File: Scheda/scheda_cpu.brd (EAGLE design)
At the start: 90 x 70 mm, 47 parts, among them IC2 LM380, IC3 AMS1117-3.3V, T1 BC-817, T2 MCU80N03A, T3 MCU80N03A, T4 MCU80N03A, T5 MCU80N03A

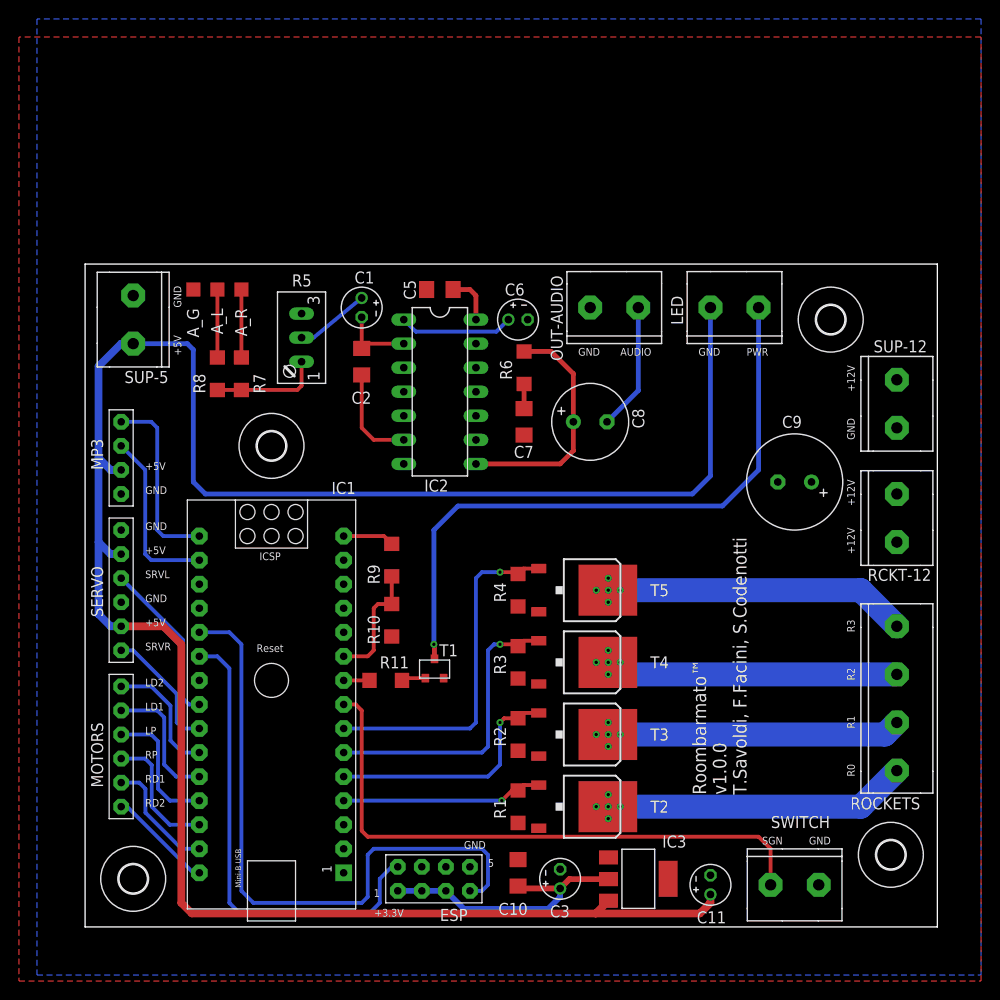
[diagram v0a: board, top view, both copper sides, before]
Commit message: completato PCB
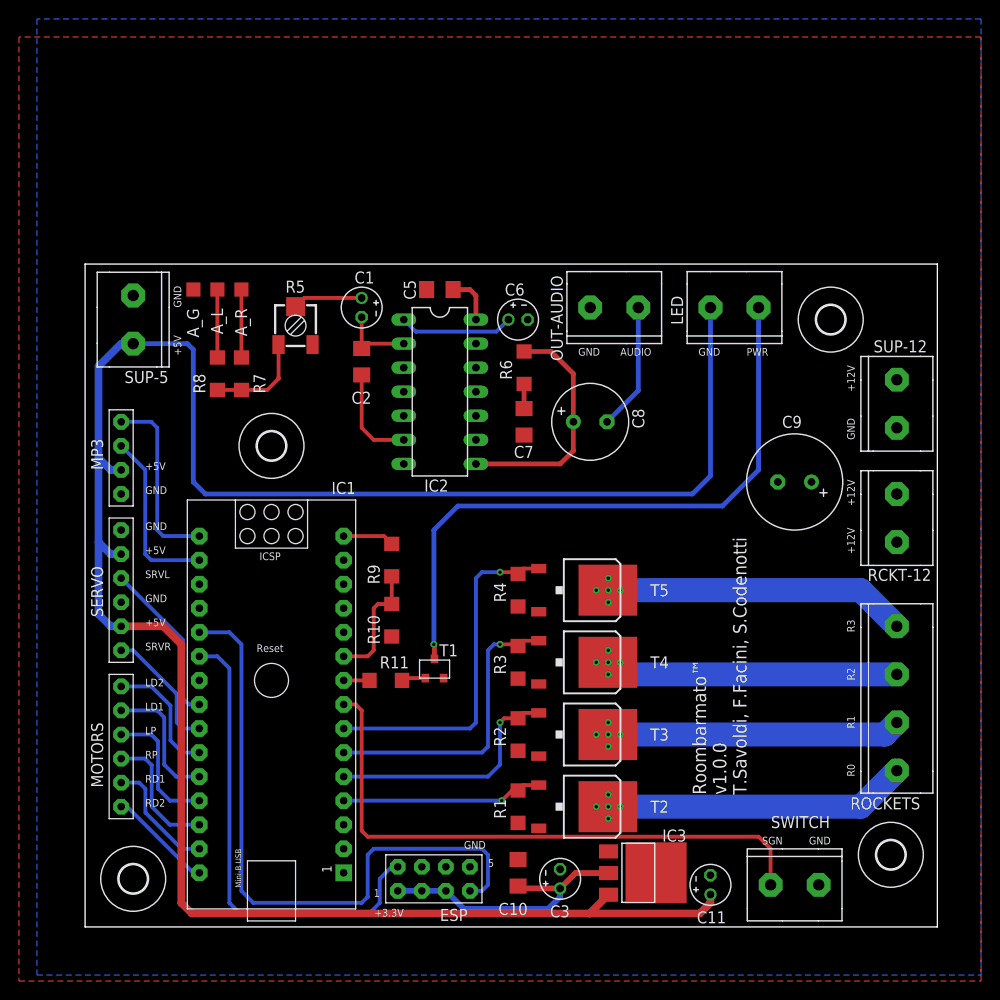
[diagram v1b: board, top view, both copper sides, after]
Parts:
- R5: value 100k -> 50k; device pot:S64W -> rcl:RTRIM3314J
- moved R5 1.42 mm to (22.2, 63.5), turned to 0 degrees
- moved IC3 0.63 mm to (58.4, 5.71)
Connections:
- net GND: now also R5.1; no longer R5.E
- net IN_AUDIO: now also R5.3; no longer R5.A
- net N$5: now also R5.2; no longer R5.S
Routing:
- net IN_AUDIO: track 11.6 -> 10.6 mm
- net +5V: track 227.9 -> 228.8 mm
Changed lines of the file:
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@@
 <grid distance="25" unitdist="mil" unit="mil" style="lines" multiple="1" display="yes" altdistance="5" altunitdist="mil" altunit="mil"/>
 <layers>
-<layer number="1" name="Top" color="4" fill="1" visible="no" active="yes"/>
-<layer number="16" name="Bottom" color="1" fill="1" visible="no" active="yes"/>
+<layer number="1" name="Top" color="4" fill="1" visible="yes" active="yes"/>
+<layer number="16" name="Bottom" color="1" fill="1" visible="yes" active="yes"/>
 <layer number="17" name="Pads" color="2" fill="1" visible="yes" active="yes"/>
 <layer number="18" name="Vias" color="2" fill="1" visible="yes" active="yes"/>
@@
 <layer number="25" name="tNames" color="7" fill="1" visible="yes" active="yes"/>
 <layer number="26" name="bNames" color="7" fill="1" visible="yes" active="yes"/>
-<layer number="27" name="tValues" color="7" fill="1" visible="yes" active="yes"/>
-<layer number="28" name="bValues" color="7" fill="1" visible="yes" active="yes"/>
-<layer number="29" name="tStop" color="7" fill="3" visible="yes" active="yes"/>
-<layer number="30" name="bStop" color="7" fill="6" visible="yes" active="yes"/>
+<layer number="27" name="tValues" color="7" fill="1" visible="no" active="yes"/>
+<layer number="28" name="bValues" color="7" fill="1" visible="no" active="yes"/>
+<layer number="29" name="tStop" color="7" fill="3" visible="no" active="yes"/>
+<layer number="30" name="bStop" color="7" fill="6" visible="no" active="yes"/>
 <layer number="31" name="tCream" color="7" fill="4" visible="no" active="yes"/>
 <layer number="32" name="bCream" color="7" fill="5" visible="no" active="yes"/>
@@
 <layer number="42" name="bRestrict" color="1" fill="10" visible="yes" active="yes"/>
 <layer number="43" name="vRestrict" color="2" fill="10" visible="no" active="yes"/>
-<layer number="44" name="Drills" color="7" fill="1" visible="yes" active="yes"/>
+<layer number="44" name="Drills" color="7" fill="1" visible="no" active="yes"/>
 <layer number="45" name="Holes" color="7" fill="1" visible="no" active="yes"/>
 <layer number="46" name="Milling" color="3" fill="1" visible="no" active="yes"/>
@@
 <text x="40.005" y="8.255" size="0.8128" layer="25">GND</text>
 <text x="81.28" y="31.115" size="0.8128" layer="25" rot="R90">R3</text>
-<polygon width="0.1524" layer="17">
-<vertex x="57.785" y="7.62"/>
-<vertex x="57.785" y="2.54"/>
-<vertex x="63.5" y="2.54"/>
-<vertex x="63.5" y="7.62"/>
-</polygon>
 <text x="52.07" y="60.325" size="0.8128" layer="25">GND</text>
 <text x="64.77" y="60.325" size="0.8128" layer="25">GND</text>
@@
 <attribute name="NAME" x="35.814" y="45.974" size="1.27" layer="25" ratio="10"/>
 </element>
-<element name="R5" library="pot" library_urn="urn:adsk.eagle:library:331" package="S64W" package3d_urn="urn:adsk.eagle:package:22708/1" value="100k" x="21.59" y="62.23" smashed="yes" rot="R270">
-<attribute name="NAME" x="21.844" y="67.6402" size="1.27" layer="25" ratio="10"/>
-<attribute name="POPULARITY" value="4" x="21.59" y="62.23" size="1.778" layer="27" rot="R270" display="off"/>
+<element name="R5" library="rcl" library_urn="urn:adsk.eagle:library:334" package="RTRIM3314J" package3d_urn="urn:adsk.eagle:package:26019/1" value="50k" x="22.225" y="63.5" smashed="yes">
+<attribute name="NAME" x="23.241" y="68.2498" size="1.27" layer="25" ratio="10" rot="R180"/>
+<attribute name="POPULARITY" value="0" x="22.225" y="63.5" size="1.778" layer="27" display="off"/>
+<attribute name="SPICEMODEL" value="X" x="22.225" y="63.5" size="1.778" layer="27" display="off"/>
+<attribute name="SPICEPREFIXL" value="POT" x="22.225" y="63.5" size="1.778" layer="27" display="off"/>
 </element>
 <element name="C1" library="ITIS" package="E2-4" value="10uF" x="29.21" y="65.405" smashed="yes" rot="R270">
@@
 </element>
 <element name="H4" library="ITIS" package="3,0" value="MOUNT-HOLE3.0" x="85.09" y="7.62" smashed="yes"/>
-<element name="IC3" library="roombarmato_eagle_lib" package="SOT223" package3d_urn="urn:adsk.eagle:package:4940/1" value="AMS1117-3.3V" x="58.42" y="5.08" smashed="yes" rot="R270">
-<attribute name="MF" value="" x="58.42" y="5.08" size="1.778" layer="27" rot="R270" display="off"/>
-<attribute name="MPN" value="REG1117" x="58.42" y="5.08" size="1.778" layer="27" rot="R270" display="off"/>
-<attribute name="NAME" x="63.5" y="9.652" size="1.27" layer="25" ratio="10" rot="R180"/>
-<attribute name="OC_FARNELL" value="1097566" x="58.42" y="5.08" size="1.778" layer="27" rot="R270" display="off"/>
-<attribute name="OC_NEWARK" value="14P6981" x="58.42" y="5.08" size="1.778" layer="27" rot="R270" display="off"/>
-<attribute name="POPULARITY" value="49" x="58.42" y="5.08" size="1.778" layer="27" rot="R270" display="off"/>
+<element name="IC3" library="roombarmato_eagle_lib" package="SOT223" package3d_urn="urn:adsk.eagle:package:4940/1" value="AMS1117-3.3V" x="58.42" y="5.715" smashed="yes" rot="R270">
+<attribute name="MF" value="" x="58.42" y="5.715" size="1.778" layer="27" rot="R270" display="off"/>
+<attribute name="MPN" value="REG1117" x="58.42" y="5.715" size="1.778" layer="27" rot="R270" display="off"/>
+<attribute name="NAME" x="63.5" y="10.287" size="1.27" layer="25" ratio="10" rot="R180"/>
+<attribute name="OC_FARNELL" value="1097566" x="58.42" y="5.715" size="1.778" layer="27" rot="R270" display="off"/>
+<attribute name="OC_NEWARK" value="14P6981" x="58.42" y="5.715" size="1.778" layer="27" rot="R270" display="off"/>
+<attribute name="POPULARITY" value="49" x="58.42" y="5.715" size="1.778" layer="27" rot="R270" display="off"/>
 </element>
 <element name="C10" library="ITIS" package="C1206" value="100nF" x="45.72" y="5.715" smashed="yes" rot="R90">
@@
 <contactref element="R1" pad="P$1"/>
 <contactref element="IC2" pad="5"/>
-<contactref element="R5" pad="E"/>
+<contactref element="R5" pad="1"/>
 <contactref element="C6" pad="-"/>
 <contactref element="C5" pad="2"/>
@@
 <wire x1="10.16" y1="2.54" x2="11.2776" y2="1.4224" width="0.8128" layer="1"/>
 <contactref element="IC3" pad="3"/>
-<wire x1="55.2704" y1="2.7686" x2="53.9242" y2="1.4224" width="0.8128" layer="1"/>
-<wire x1="11.2776" y1="1.4224" x2="53.9242" y2="1.4224" width="0.8128" layer="1"/>
-<wire x1="53.9242" y1="1.4224" x2="64.9224" y2="1.4224" width="0.8128" layer="1"/>
+<wire x1="55.2704" y1="3.4036" x2="53.2892" y2="1.4224" width="0.8128" layer="1"/>
+<wire x1="11.2776" y1="1.4224" x2="53.2892" y2="1.4224" width="0.8128" layer="1"/>
+<wire x1="53.2892" y1="1.4224" x2="64.9224" y2="1.4224" width="0.8128" layer="1"/>
 <contactref element="C11" pad="+"/>
 <wire x1="64.9224" y1="1.4224" x2="66.04" y2="2.54" width="0.8128" layer="1"/>
@@
 <contactref element="IC3" pad="2"/>
 <wire x1="40.005" y1="1.905" x2="48.895" y2="1.905" width="0.6096" layer="16"/>
-<wire x1="51.1556" y1="5.0546" x2="55.2704" y2="5.0546" width="0.6096" layer="1"/>
+<wire x1="51.7906" y1="5.6896" x2="55.2704" y2="5.6896" width="0.6096" layer="1"/>
 <contactref element="C10" pad="1"/>
 <contactref element="C3" pad="+"/>
-<wire x1="50.165" y1="4.064" x2="51.1556" y2="5.0546" width="0.6096" layer="1"/>
+<wire x1="50.165" y1="4.064" x2="51.7906" y2="5.6896" width="0.6096" layer="1"/>
 <wire x1="48.895" y1="1.905" x2="50.165" y2="3.175" width="0.6096" layer="16"/>
 <wire x1="50.165" y1="3.175" x2="50.165" y2="4.064" width="0.6096" layer="16"/>
@@
 </signal>
 <signal name="IN_AUDIO">
-<contactref element="R5" pad="A"/>
+<contactref element="R5" pad="3"/>
 <contactref element="R7" pad="P$2"/>
 <contactref element="R8" pad="P$2"/>
-<wire x1="22.86" y1="57.15" x2="22.4155" y2="56.7055" width="0.4064" layer="1"/>
-<wire x1="22.86" y1="57.15" x2="22.86" y2="59.69" width="0.4064" layer="1"/>
-<wire x1="22.4155" y1="56.7055" x2="16.51" y2="56.7055" width="0.4064" layer="1"/>
+<wire x1="20.45055625" y1="57.91555625" x2="19.2405" y2="56.7055" width="0.4064" layer="1"/>
+<wire x1="20.45055625" y1="57.91555625" x2="20.425" y2="57.9612125" width="0.4064" layer="1"/>
+<wire x1="20.425" y1="57.9612125" x2="20.425" y2="61.5" width="0.4064" layer="1"/>
+<wire x1="19.2405" y1="56.7055" x2="16.51" y2="56.7055" width="0.4064" layer="1"/>
 <wire x1="16.51" y1="56.7055" x2="13.97" y2="56.7055" width="0.4064" layer="1"/>
 </signal>
 <signal name="N$5">
-<contactref element="R5" pad="S"/>
+<contactref element="R5" pad="2"/>
 <contactref element="C1" pad="+"/>
-<wire x1="29.21" y1="66.421" x2="24.13" y2="62.23" width="0.4064" layer="16"/>
-<wire x1="22.86" y1="62.23" x2="24.13" y2="62.23" width="0.4064" layer="16"/>
+<wire x1="22.225" y1="65.5" x2="23.146" y2="66.421" width="0.4064" layer="1"/>
+<wire x1="23.146" y1="66.421" x2="29.21" y2="66.421" width="0.4064" layer="1"/>
 </signal>
 <signal name="N$6">
@@
 </signals>
 <mfgpreviewcolors>
-<mfgpreviewcolor name="soldermaskcolor" color="0xC8008000"/>
+<mfgpreviewcolor name="soldermaskcolor" color="0xC8FF00FF"/>
 <mfgpreviewcolor name="silkscreencolor" color="0xFFFEFEFE"/>
 <mfgpreviewcolor name="backgroundcolor" color="0xFF282828"/>
